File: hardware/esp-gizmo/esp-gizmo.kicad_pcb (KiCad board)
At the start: 2 copper layers, 27 parts, among them P1 CONN_01X04, P2 CONN_01X02, P3 CONN_01X03, P4 BOOT JUMPER, P5 CONN_01X04, SW1 SPST, U1 AC-DC, U2 ESP-12E, U3 MOC3021S, U4 MOC3021S, U5 MOC3021S, U6 TRIAC, U7 TRIAC, U8 TRIAC

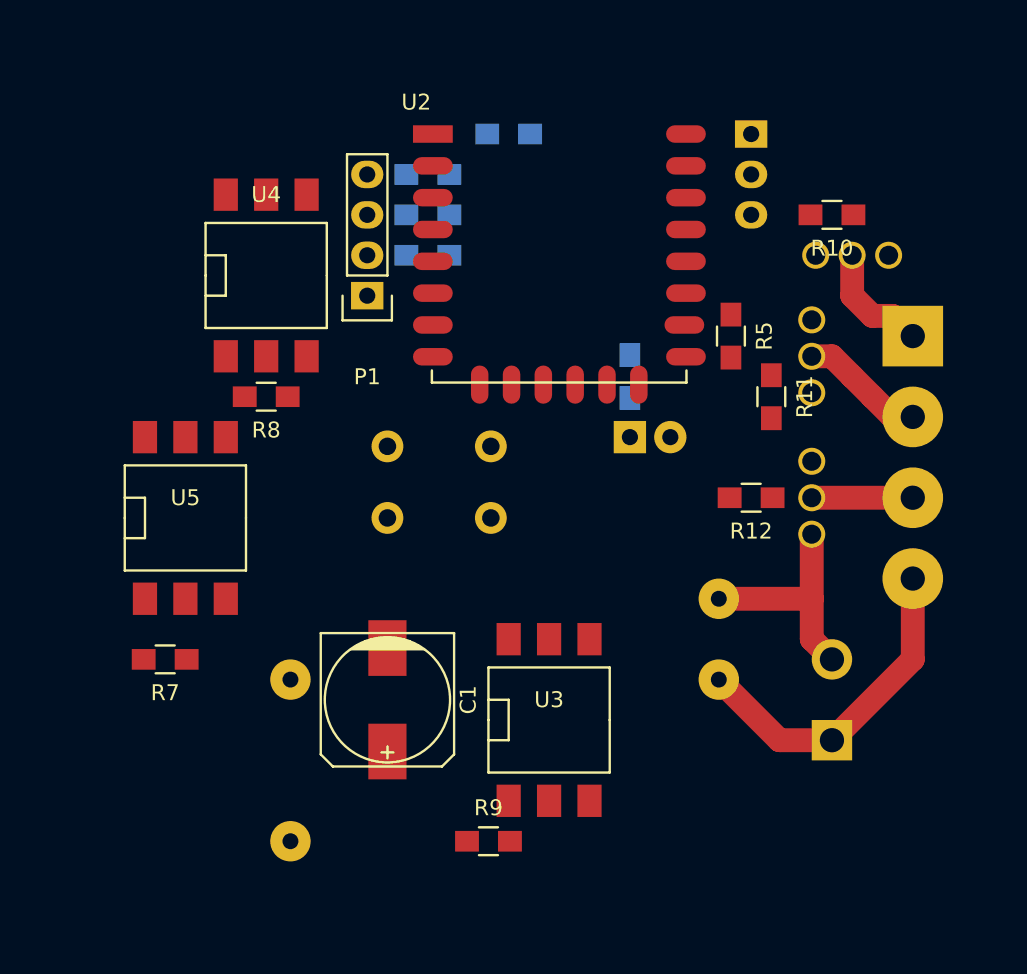
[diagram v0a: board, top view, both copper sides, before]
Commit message: Draft pcb design
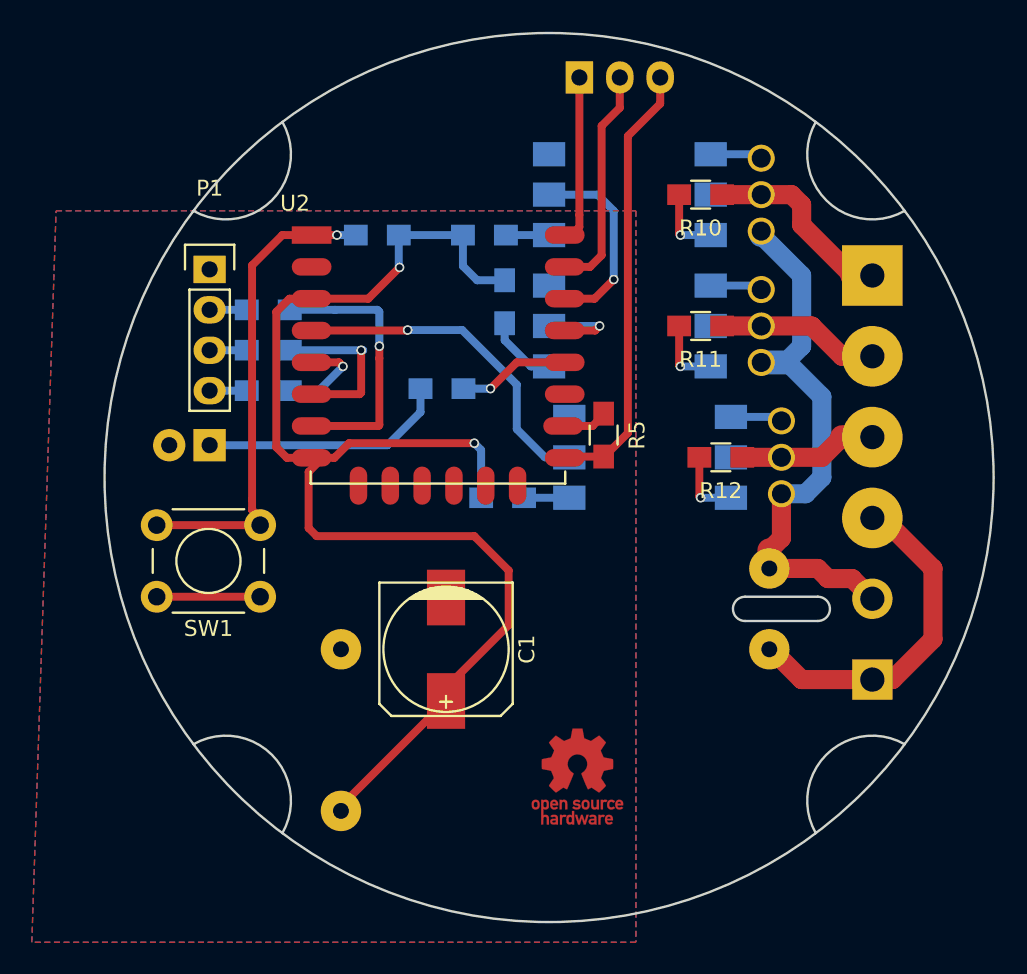
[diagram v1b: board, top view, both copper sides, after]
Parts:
- added REF***: OSHW-Logo_5.7x6mm_Copper, Symbols:OSHW-Logo_5.7x6mm_Copper, F.Cu at (136.4, 130.6)
- R7, R8, R9, U3, U4, U5: moved to B.Cu
- SW1: moved to F.Cu
- moved R9 38.1 mm to (130.6, 96.5)
- moved U3 33.4 mm to (139.7, 94.0), turned to 90 degrees
- moved U5 29.5 mm to (141.0, 110.5), turned to 90 degrees
- moved P4 26.4 mm to (113.3, 109.7), turned to 90 degrees
- moved R7 23.5 mm to (131.7, 113.0), turned to 0 degrees
- moved U4 23.1 mm to (139.7, 102.2), turned to 90 degrees
- moved R1 16.9 mm to (117.0, 106.3)
- moved R8 16.1 mm to (131.8, 100.7), turned to 270 degrees
- moved R2 13.2 mm to (117.0, 103.8)
- moved R6 11.8 mm to (127.9, 106.2), turned to 0 degrees
- moved P3 11.4 mm to (136.5, 86.6), turned to 270 degrees
- moved R3 10.6 mm to (117.0, 101.2)
- moved R4 10.4 mm to (123.8, 96.5)
- moved R5 10.1 mm to (138.0, 109.1)
- moved P1 10.0 mm to (113.3, 98.7), turned to 0 degrees
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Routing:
- net +3V3: track 0.00 -> 83.1 mm, vias 0 -> 2
- net GND: track 0.00 -> 35.3 mm
- net Net-(R4-Pad2): track 0.00 -> 30.4 mm, vias 0 -> 1
- net Net-(P2-Pad2): track 14.2 -> 36.3 mm
- net Net-(U2-Pad4): track 0.00 -> 20.5 mm, vias 0 -> 1
- net Net-(R3-Pad1): track 0.00 -> 16.4 mm, vias 0 -> 1
- net Net-(P4-Pad1): track 0.00 -> 15.6 mm
- net Net-(P3-Pad2): track 0.00 -> 15.0 mm
- net Net-(U2-Pad20): track 0.00 -> 13.1 mm, vias 0 -> 1
- net Net-(P3-Pad1): track 0.00 -> 11.2 mm
- net Net-(R2-Pad1): track 0.00 -> 10.00 mm, vias 0 -> 1
- net Net-(R6-Pad2): track 0.00 -> 6.35 mm, vias 0 -> 1
- net Net-(U2-Pad19): track 0.00 -> 6.18 mm, vias 0 -> 1
- net Net-(R1-Pad1): track 0.00 -> 5.36 mm, vias 0 -> 1
- net /LOAD_1: track 7.40 -> 12.3 mm
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- added copper zone on B.Cu, net GND
- added copper zone on F.Cu, net GND
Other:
- board outline added: 55.9 x 55.9 mm
- net class Default: trace_width 0.25 -> 0.5
- net class hi_voltage added: clearance 0.5, trace_width 0.5, via_dia 0.6, via_drill 0.4
- net class load: trace_width 1.5 -> 1.2
